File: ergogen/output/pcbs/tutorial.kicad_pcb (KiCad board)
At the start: 2 copper layers, 134 x 91.6 mm, 44 parts

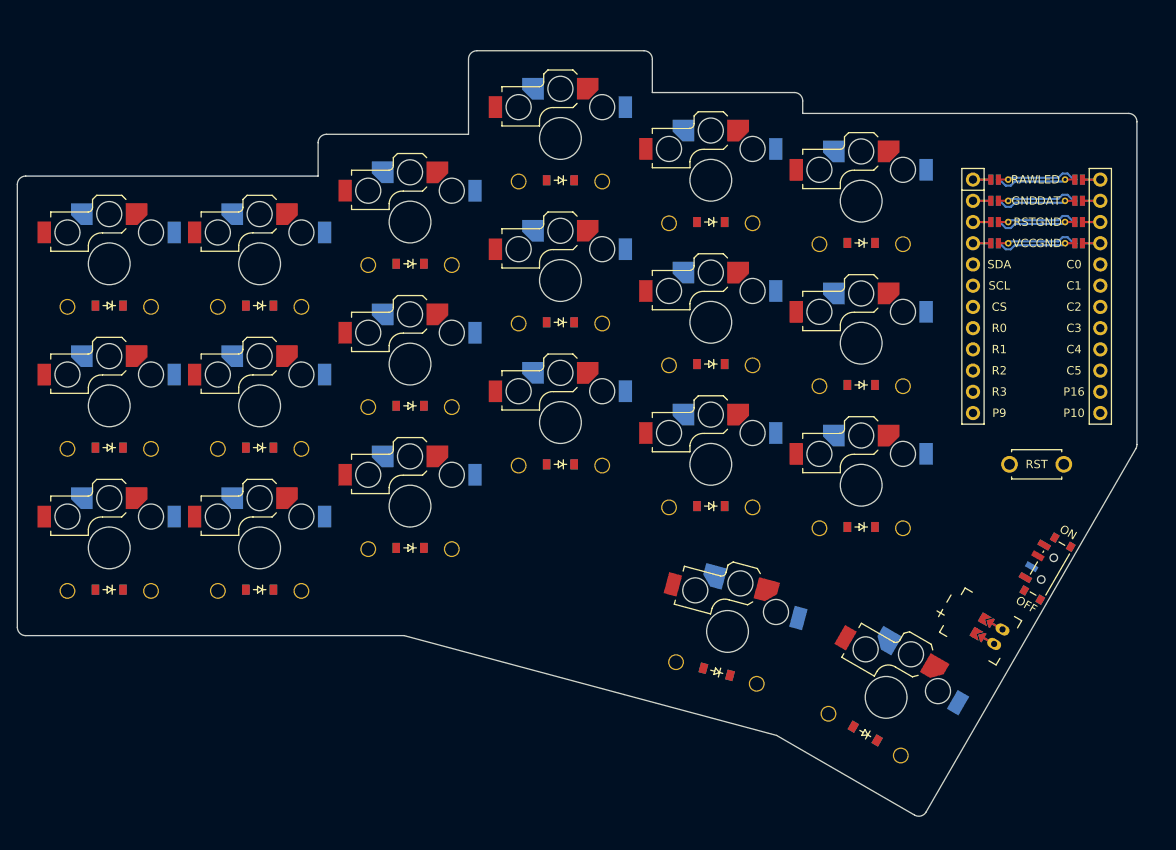
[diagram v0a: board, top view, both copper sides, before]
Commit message: feat: ceoloide suggestions
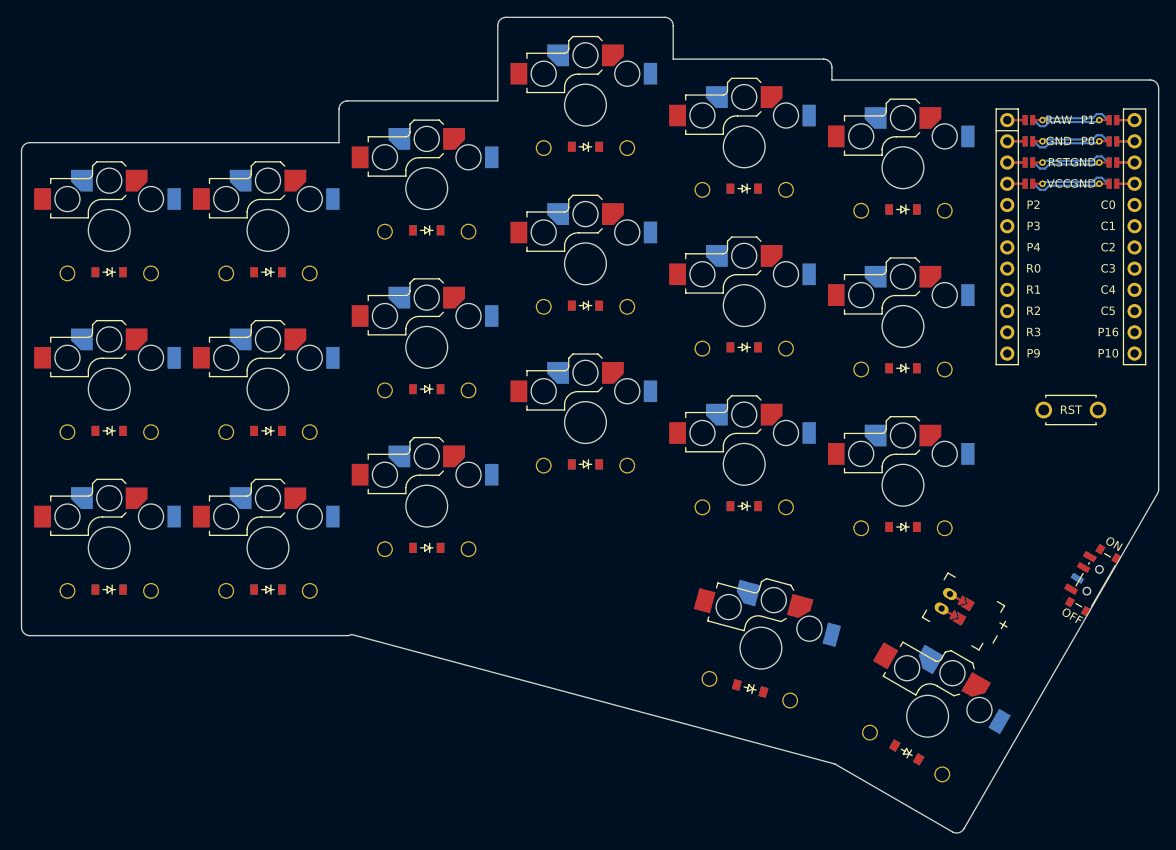
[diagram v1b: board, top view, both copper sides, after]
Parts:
- moved MCU1 8.22 mm to (215.1, 61.5)
- moved RST1 7.69 mm to (215.1, 83.5)
- moved JST1 7.59 mm to (200.1, 106.4), turned to 60 degrees
- moved D18 6.40 mm to (195.0, 59.5)
- moved S18 6.40 mm to (195.0, 54.5)
- moved D15 5.66 mm to (176.0, 57.0)
- moved S15 5.66 mm to (176.0, 52.0)
- moved PWR1 5.64 mm to (217.7, 103.9)
- moved D20 5.46 mm to (195.5, 124.5)
- moved S20 5.46 mm to (198.0, 120.1)
- moved D17 5.39 mm to (195.0, 78.5)
- moved S17 5.39 mm to (195.0, 73.5)
- moved D12 5.00 mm to (157.0, 52.0)
- moved D16 5.00 mm to (195.0, 97.5)
- moved S12 5.00 mm to (157.0, 47.0)
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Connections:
- net CS renamed P4
- net DAT renamed P0
- net LED renamed P1
- net SCL renamed P3
- net SDA renamed P2
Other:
- board size 134 x 91.6 mm -> 136.1 x 97.6 mm
